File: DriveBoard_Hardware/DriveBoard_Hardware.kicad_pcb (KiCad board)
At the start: 2 copper layers, 61 x 91.2 mm, 12 parts, among them U1 TM4C129E_Launchpad, U2 MAX_3232, U3 OKI

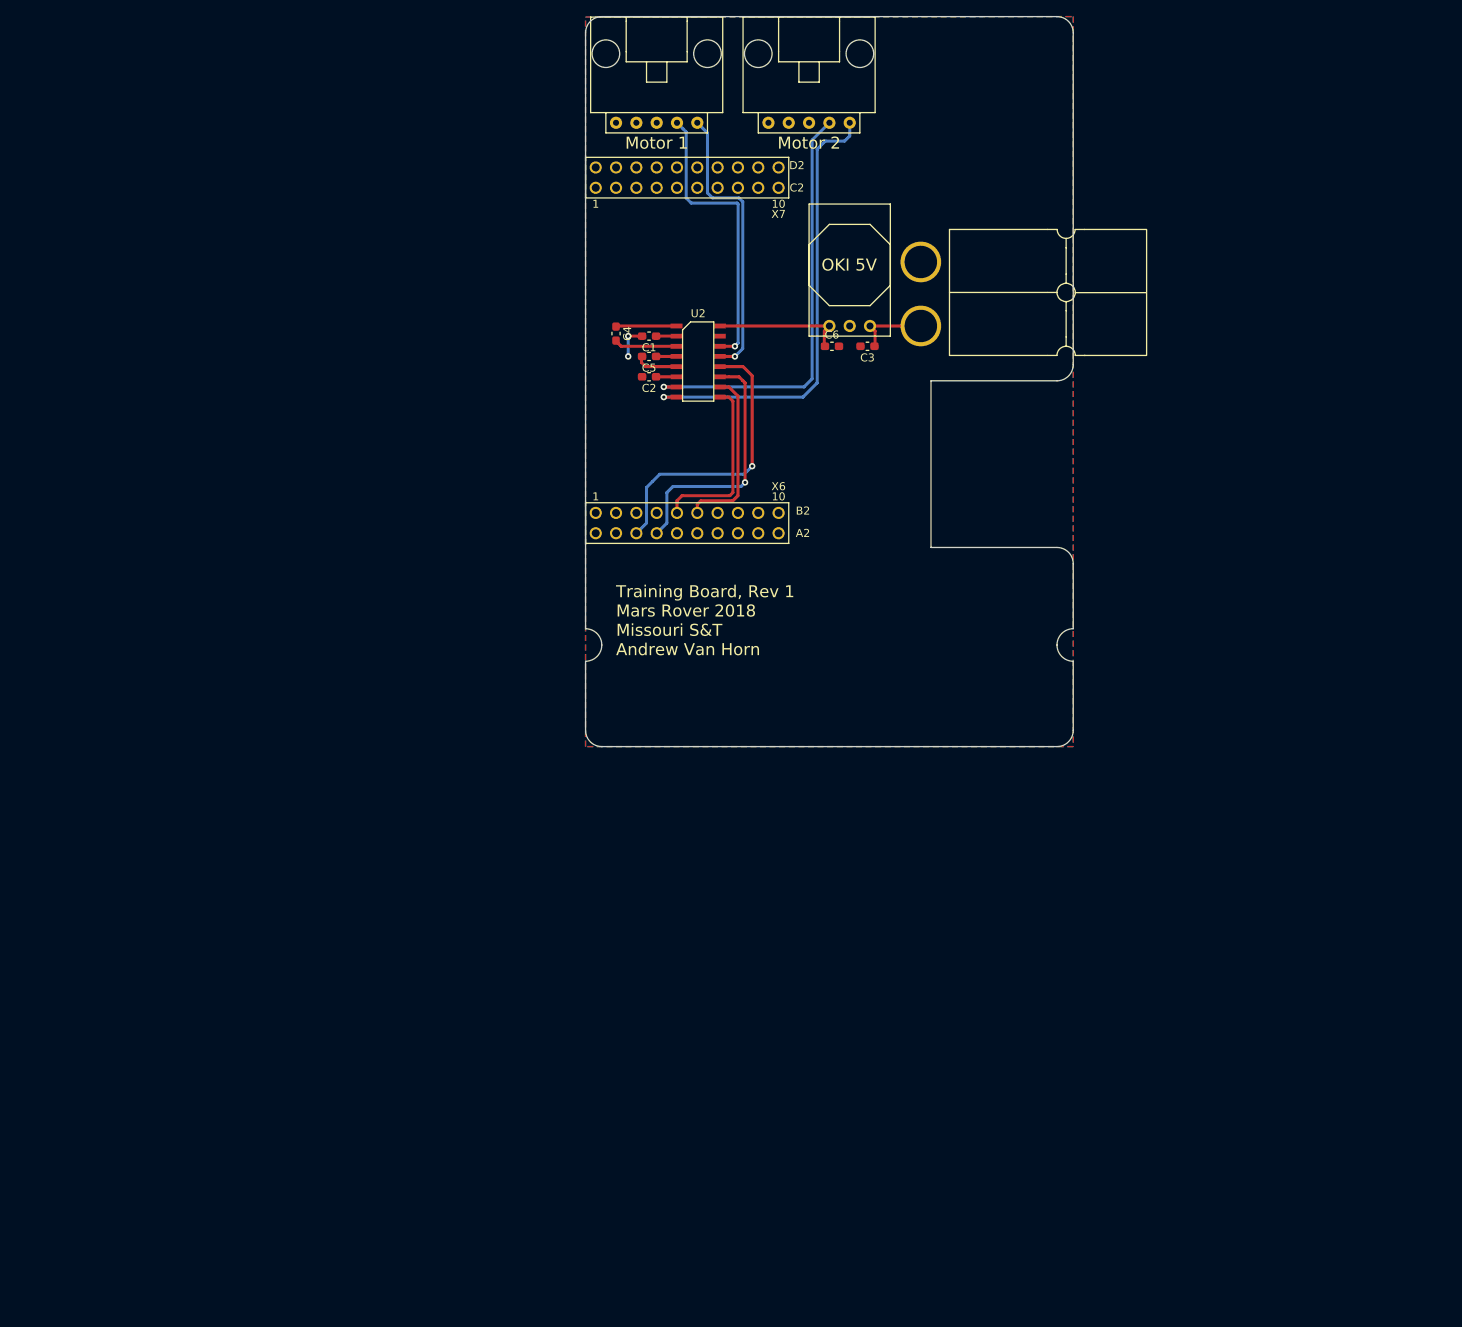
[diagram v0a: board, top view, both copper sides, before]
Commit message: Generated Gerbs and BOM
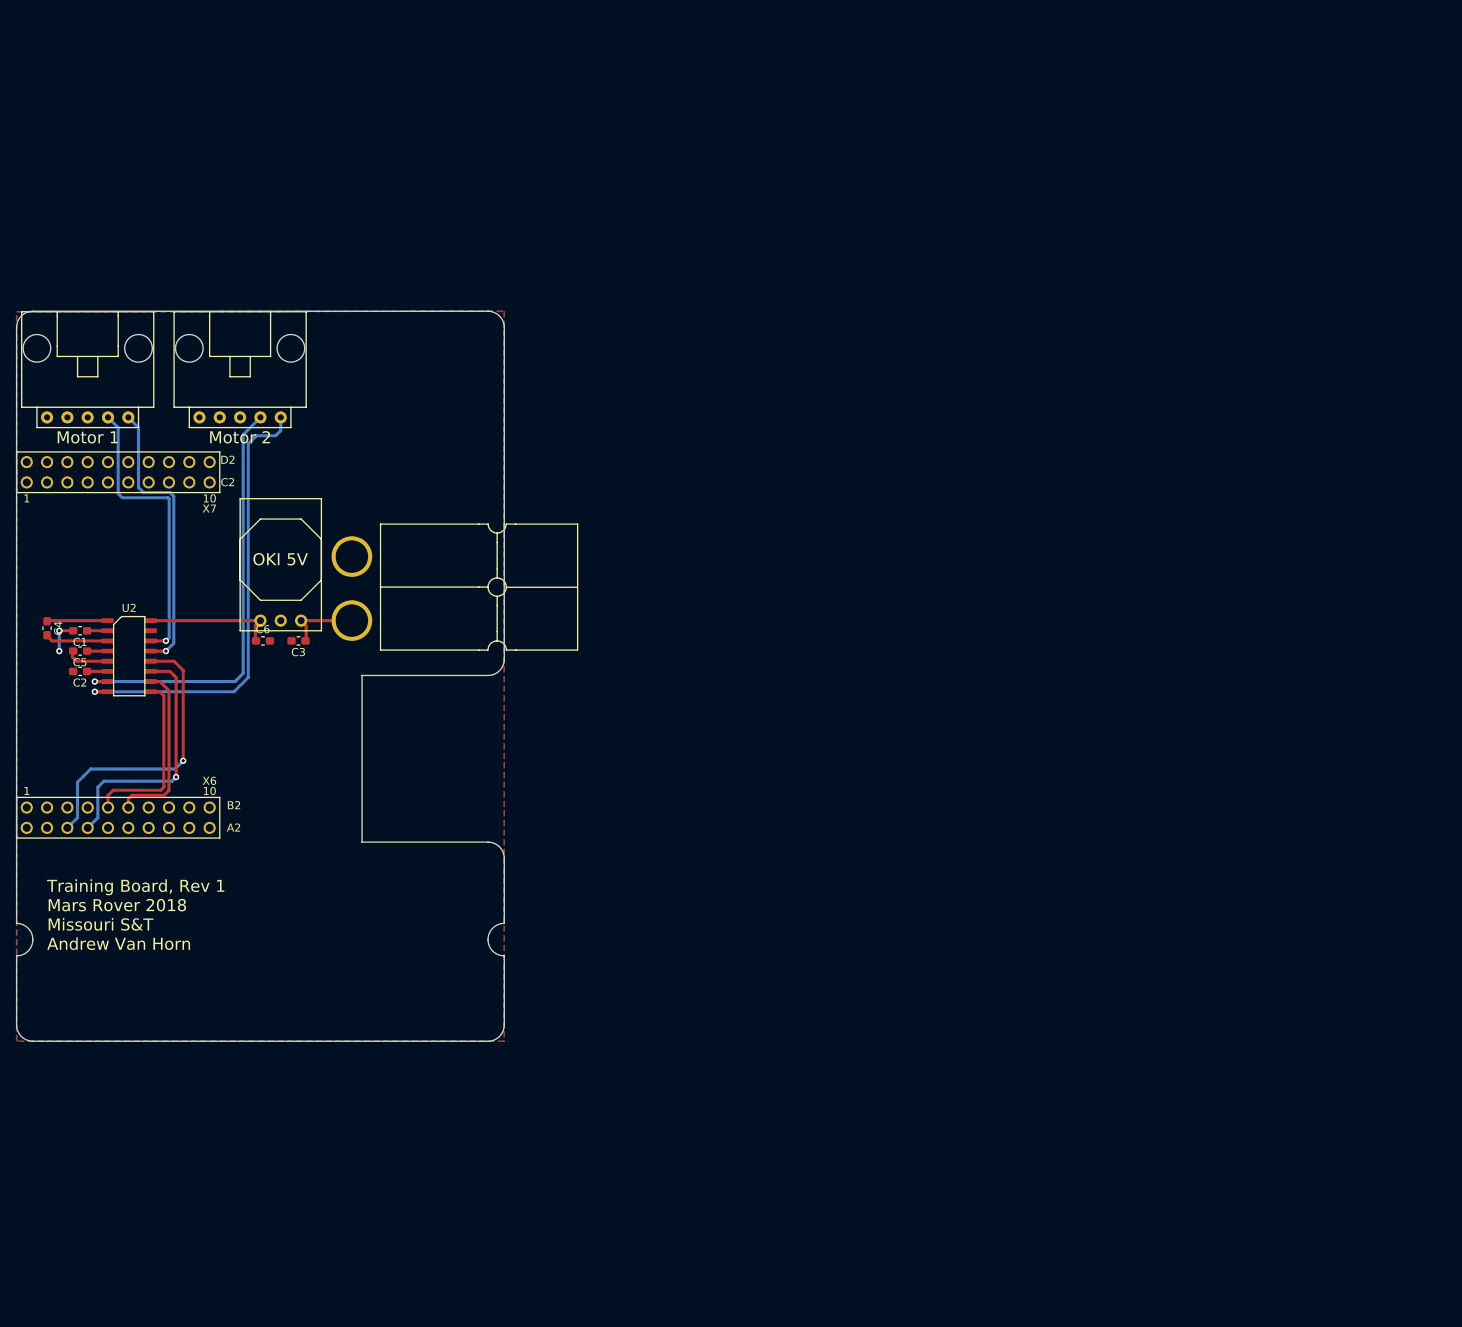
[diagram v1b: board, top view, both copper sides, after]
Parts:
- moved C2 80.1 mm to (95.6, 106.7)
- moved Conn1 80.1 mm to (133.1, 88.3)
- moved Conn3 80.1 mm to (115.6, 74.9)
- moved C1 80.1 mm to (95.6, 101.6)
- moved C3 80.1 mm to (122.9, 102.9)
- moved C4 80.1 mm to (91.4, 101.3)
- moved C5 80.1 mm to (95.6, 104.1)
- moved C6 80.1 mm to (118.4, 102.9)
- moved Conn2 80.1 mm to (96.5, 74.9)
- moved U1 80.1 mm to (87.6, 127.5)
- moved U2 80.1 mm to (101.7, 104.8)
- moved U3 80.1 mm to (125.7, 101.6)

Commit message: Board Layout Completed
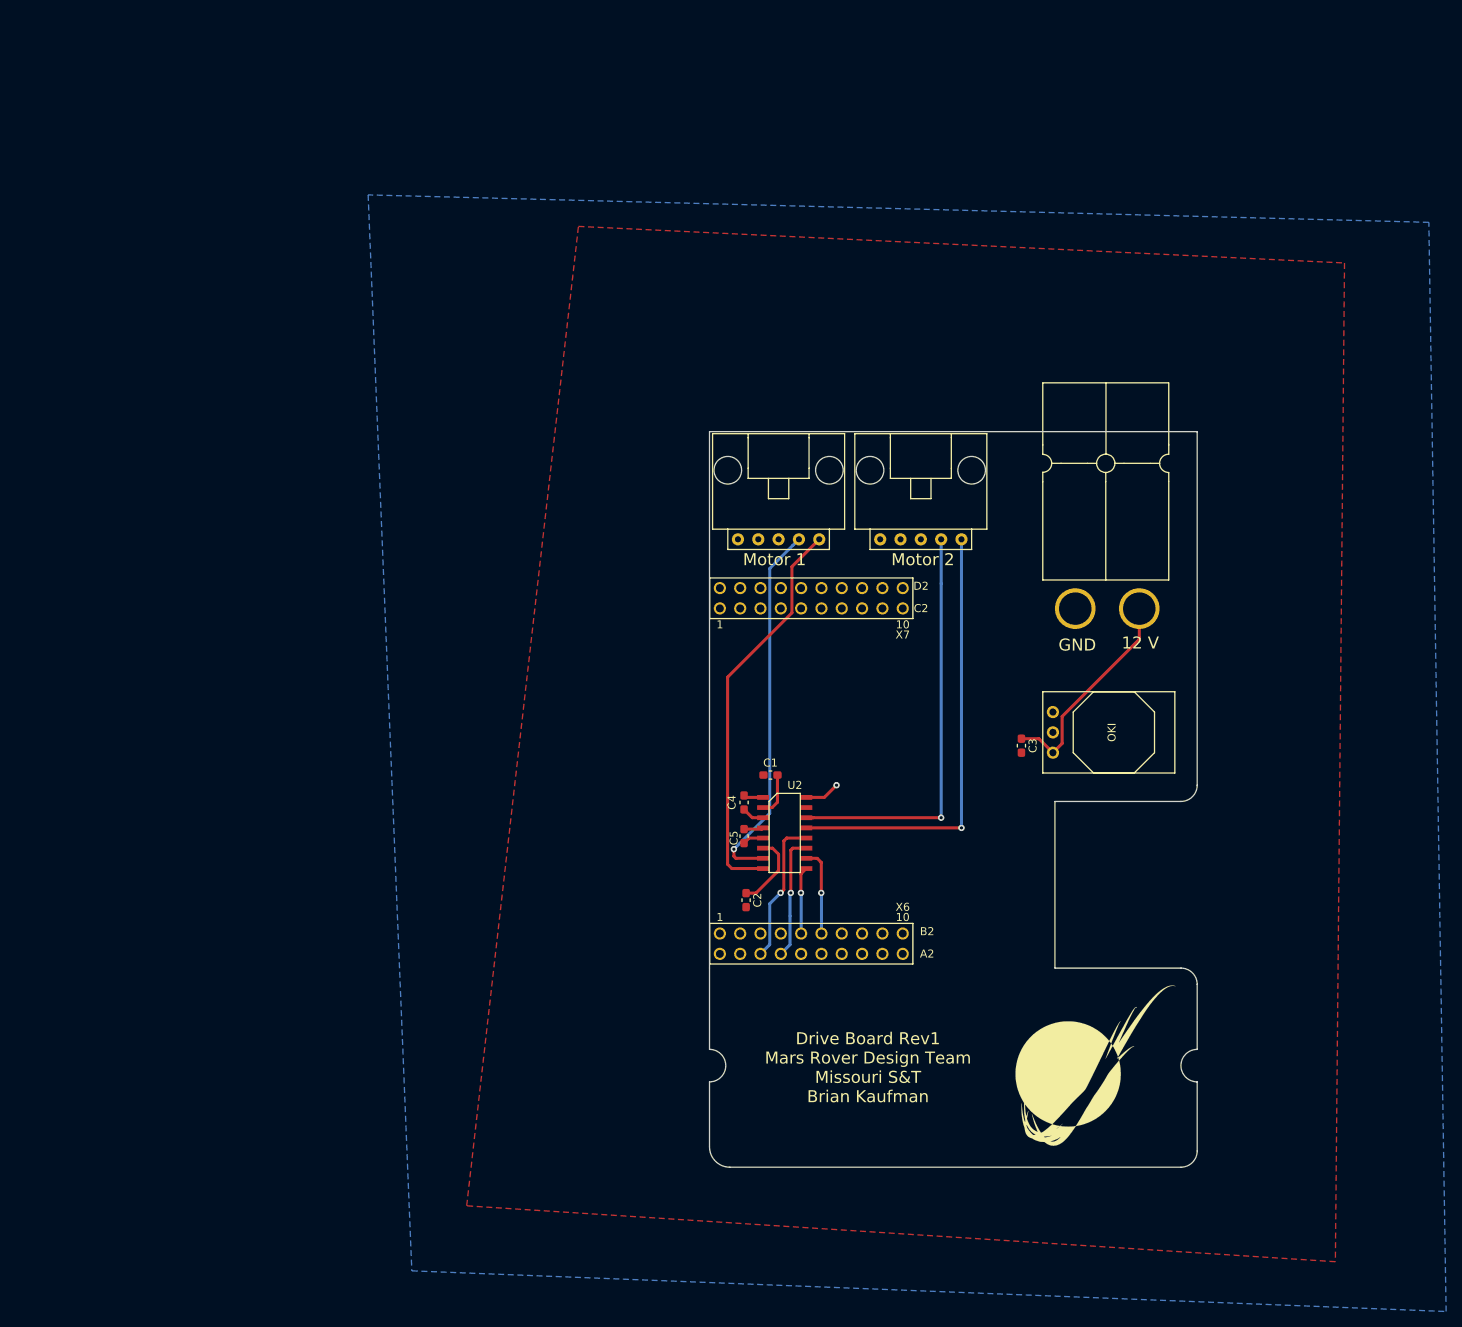
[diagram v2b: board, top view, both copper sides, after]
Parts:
- removed C6: 10uF, Capacitor_SMD:C_0603_1608Metric_Pad1.05x0.95mm_HandSolder
- added G***: LOGO, MRDT_Silkscreens:MRDT_Logo_20mm, F.Cu at (222.5, 156.0)
- moved Conn2 105.2 mm to (200.7, 90.2)
- moved U3 91.9 mm to (215.9, 119.4), turned to 90 degrees
- moved C3 91.3 mm to (213.2, 116.0), turned to 270 degrees
- moved C4 89.8 mm to (178.6, 123.1)
- moved C1 88.2 mm to (181.9, 119.6)
- moved U1 88.1 mm to (174.3, 143.3)
- moved C2 88.0 mm to (178.8, 135.3), turned to 270 degrees
- moved C5 86.2 mm to (178.6, 127.3), turned to 270 degrees
- moved U2 84.9 mm to (183.6, 126.9)
- moved Conn1 83.1 mm to (215.9, 95.2), turned to 270 degrees
- moved Conn3 69.0 mm to (182.9, 90.2)
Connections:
- Conn2 pad 1: (no net) -> Net-(Conn2-Pad1)
- Conn2 pad 2: (no net) -> Net-(Conn2-Pad2)
- Conn3 pad 1: (no net) -> Net-(Conn3-Pad1)
- Conn3 pad 2: (no net) -> Net-(Conn3-Pad2)
- U1 pad +3V3: (no net) -> Net-(U1-Pad+3V3)
- U1 pad PA4: (no net) -> Net-(U1-PadPA4)
- U1 pad PA5: (no net) -> Net-(U1-PadPA5)
- U1 pad PA7: (no net) -> Net-(U1-PadPA7)
- U1 pad PB4: (no net) -> Net-(U1-PadPB4)
- U1 pad PB5: (no net) -> Net-(U1-PadPB5)
- U1 pad PD2: (no net) -> Net-(U1-PadPD2)
- U1 pad PD4: (no net) -> Net-(U1-PadPD4)
- U1 pad PD5: (no net) -> Net-(U1-PadPD5)
- U1 pad PG1: (no net) -> Net-(U1-PadPG1)
- U1 pad PH0: (no net) -> Net-(U1-PadPH0)
- U1 pad PH1: (no net) -> Net-(U1-PadPH1)
- U1 pad PK2: (no net) -> Net-(U1-PadPK2)
- U1 pad PK3: (no net) -> Net-(U1-PadPK3)
- U1 pad PK4: (no net) -> Net-(U1-PadPK4)
- U1 pad PK5: (no net) -> Net-(U1-PadPK5)
- U1 pad PK6: (no net) -> Net-(U1-PadPK6)
- U1 pad PK7: (no net) -> Net-(U1-PadPK7)
- U1 pad PM0: (no net) -> Net-(U1-PadPM0)
- U1 pad PM1: (no net) -> Net-(U1-PadPM1)
- U1 pad PM2: (no net) -> Net-(U1-PadPM2)
- U1 pad PM6: (no net) -> Net-(U1-PadPM6)
- U1 pad PM7: (no net) -> Net-(U1-PadPM7)
- U1 pad PN4: (no net) -> Net-(U1-PadPN4)
- U1 pad PN5: (no net) -> Net-(U1-PadPN5)
- U1 pad PP3: (no net) -> Net-(U1-PadPP3)
- U1 pad PP4: (no net) -> Net-(U1-PadPP4)
- U1 pad PP5: (no net) -> Net-(U1-PadPP5)
- U1 pad PQ0: (no net) -> Net-(U1-PadPQ0)
- U1 pad PQ1: (no net) -> Net-(U1-PadPQ1)
- U1 pad PQ2: (no net) -> Net-(U1-PadPQ2)
- U1 pad PQ3: (no net) -> Net-(U1-PadPQ3)
- U1 pad Rese: (no net) -> Net-(U1-PadRese)
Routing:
- net RX_1_SL: track 35.8 -> 55.9 mm
- net /+12V: track 9.15 -> 27.1 mm
- net RX_1_IC: track 36.4 -> 18.7 mm
- net TX_1_IC: track 31.8 -> 15.5 mm
- net TX_1_SL: track 36.5 -> 52.5 mm
- net RX_2_IC: track 22.2 -> 8.86 mm, vias 0 -> 1
- net +5V: track 16.5 -> 5.36 mm, vias 0 -> 1
- net TX_2_IC: track 21.8 -> 11.4 mm, vias 0 -> 1
- net RX_2_SL: track 57.1 -> 50.0 mm, vias 1 -> 0
- net Net-(C2-Pad1): track 2.49 -> 9.52 mm
- net TX_2_SL: track 53.5 -> 47.2 mm
- net Net-(C4-Pad1): track 7.57 -> 2.48 mm
- net Net-(C4-Pad2): track 7.83 -> 2.81 mm
- net GND: track 4.20 -> 0.41 mm, vias 2 -> 0
- net Net-(C1-Pad1): track 2.49 -> 5.47 mm
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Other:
- board size 61 x 91.2 mm -> 61 x 91.9 mm
- board text added: "12 V"
- board text added: "Drive Board Rev1 Mars Rover Design Team Missouri S&T Brian Kaufman"
- board text added: "GND"
- board text removed: "OKI 5V"
- board text removed: "Training Board, Rev 1 Mars Rover 2018 Missouri S&T Andrew Van Horn"
